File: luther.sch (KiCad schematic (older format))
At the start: 6 parts, among them J1 Conn_01x02, U1 Teensy4.0, U2 RFM95W_LoRa_Radio, U3 VHN5019_Breakout, U4 VHN5019_Breakout, U5 bno055

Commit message: misc changes
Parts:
- removed U5: bno055, NUSTARS Libs:bno055, symbol NUSTARS:bno055
- added D1: LED, symbol Device:LED
- added J2: SMART_AUDIO, symbol Connector_Generic:Conn_01x02
- added J3: SERVO_LEVER, Connector_JST:JST_PH_B3B-PH-K_1x03_P2.00mm_Vertical, symbol Connector_Generic:Conn_01x03
- added J4: SERVO_CLOCK, Connector_JST:JST_PH_B3B-PH-K_1x03_P2.00mm_Vertical, symbol Connector_Generic:Conn_01x03
- added R1: 330, symbol Device:R_Small_US
- added SW1: SW_SPST, NUSTARS Libs:GF-123-0054, symbol Switch:SW_SPST
- added U5: VHN5019_Breakout, NUSTARS Libs:VNH5019_breakout, symbol NUSTARS:VHN5019_Breakout
- added U6, U7: BUCK, symbol NUSTARS:BUCK
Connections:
- net labels added: 3V3B, M0_INA, M0_INB, M0_PWM, M1_INA, M1_INB, M1_PWM, M2_INA, M2_INB, M2_PWM
- net labels removed: FNA2T, T2FNA
- wire segments 5 -> 26
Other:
- note removed: "Consider hooking this up to 3.3V buck output\n"
- moved on the sheet: J1, U2, U3, U4

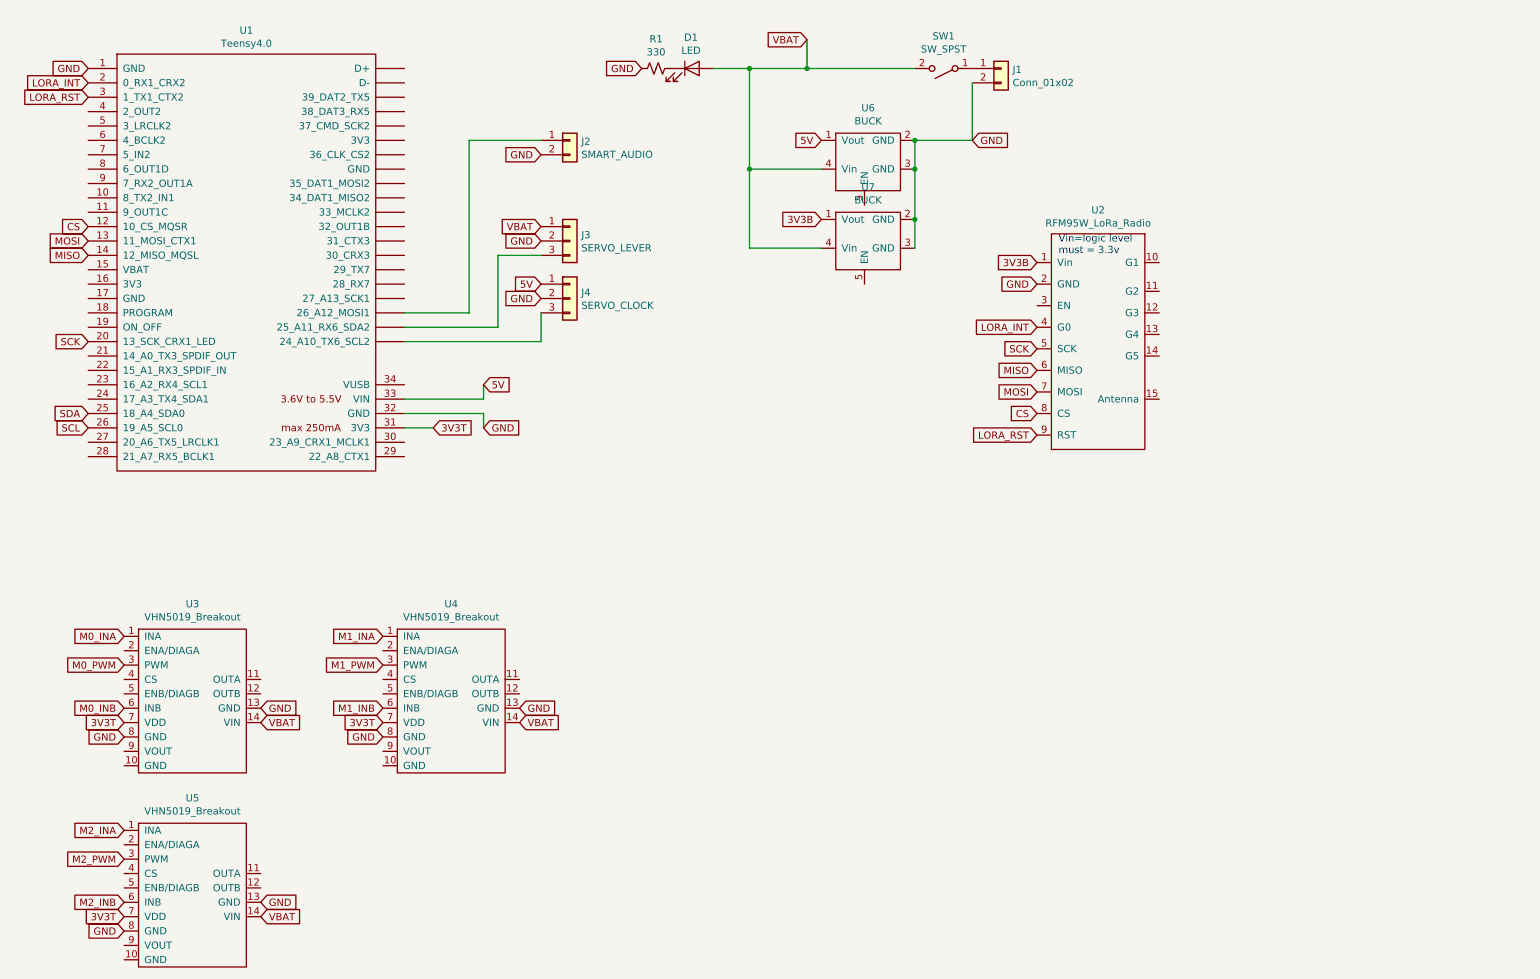
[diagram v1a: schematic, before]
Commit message: updates
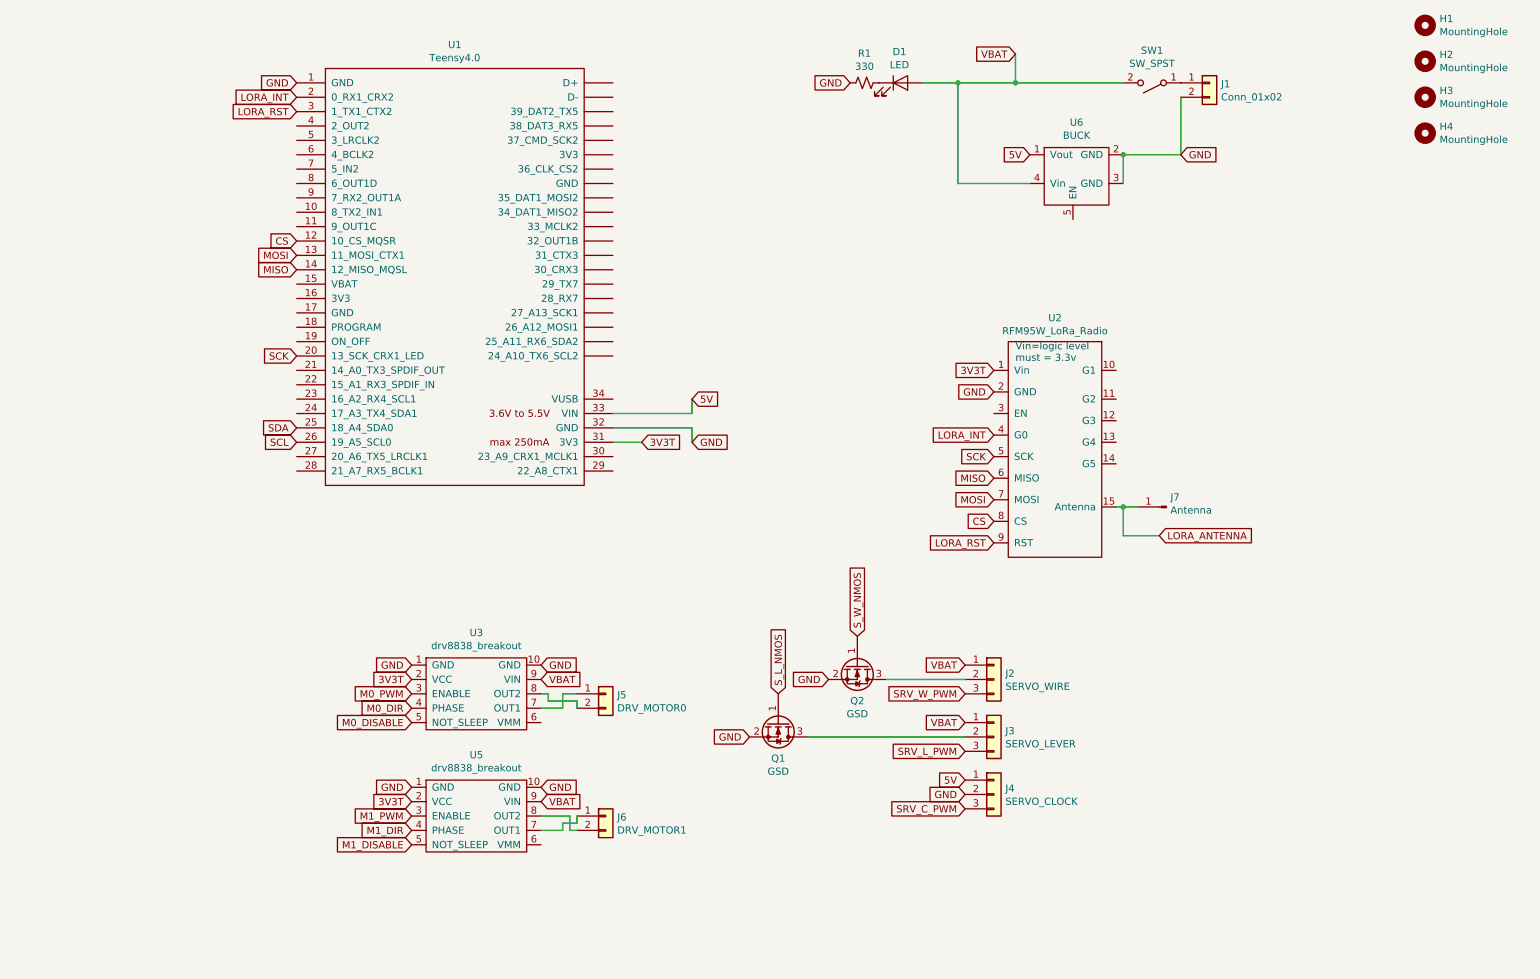
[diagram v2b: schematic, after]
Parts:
- removed J2: SMART_AUDIO, symbol Connector_Generic:Conn_01x02
- removed U3, U4, U5: VHN5019_Breakout, NUSTARS Libs:VNH5019_breakout, symbol NUSTARS:VHN5019_Breakout
- removed U7: BUCK, symbol NUSTARS:BUCK
- added H1, H2, H3, H4: MountingHole, MountingHole:MountingHole_3.2mm_M3, symbol Mechanical:MountingHole
- added J2: SERVO_WIRE, Connector_JST:JST_PH_B3B-PH-K_1x03_P2.00mm_Vertical, symbol Connector_Generic:Conn_01x03
- added J5: DRV_MOTOR0, Connector_JST:JST_PH_B2B-PH-K_1x02_P2.00mm_Vertical, symbol Connector_Generic:Conn_01x02
- added J6: DRV_MOTOR1, Connector_JST:JST_PH_B2B-PH-K_1x02_P2.00mm_Vertical, symbol Connector_Generic:Conn_01x02
- added J7: Antenna, NUSTARS Libs:Antenna, symbol Connector:Conn_01x01_Male
- added Q1, Q2: GSD, Package_TO_SOT_SMD:SOT-23_Handsoldering, symbol Device:Q_NMOS_GSD
- added U3, U5: drv8838_breakout, NUSTARS Libs:drv8838_breakout, symbol DRV:drv8838_breakout
- D1: footprint (none) -> LED_SMD:LED_1206_3216Metric_Pad1.42x1.75mm_HandSolder
- R1: footprint (none) -> Resistor_SMD:R_1206_3216Metric_Pad1.42x1.75mm_HandSolder
- U6: footprint (none) -> NUSTARS Libs:D24V50F5
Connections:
- net 3V3B is gone; now on net 3V3T: U2.1 (Vin)
- net 3V3T: now also U3.2 (VCC), U5.2 (VCC)
- net GND: now also Q1.2 (S), Q2.2 (S), U3.1 (GND), U3.10 (GND), U5.1 (GND), U5.10 (GND); no longer J3.2 (Pin_2)
- net M0_PWM: now also U3.3 (ENABLE)
- net M1_PWM: now also U5.3 (ENABLE)
- net VBAT: now also J2.1 (Pin_1), U3.9 (VIN), U5.9 (VIN)
- net SRV_L_PWM: now reaches J3.3 (Pin_3)
- net SRV_L_PWM: no longer U1.~ (GND)
- net SRV_C_PWM: now reaches J4.3 (Pin_3)
- net SRV_C_PWM: no longer U1.~ (GND)
- net LORA_ANTENNA: now reaches U2.15 (Antenna)
- net LORA_ANTENNA: now also J7.1 (Pin_1)
- new net: J6.1 (Pin_1), U5.7 (OUT1)
- new net: J6.2 (Pin_2), U5.8 (OUT2)
- new net: J5.1 (Pin_1), U3.7 (OUT1)
- new net: J5.2 (Pin_2), U3.8 (OUT2)
- new net: J3.2 (Pin_2), Q1.3 (D)
- new net: J2.2 (Pin_2), Q2.3 (D)
- new net M0_DIR: U3.4 (PHASE)
- new net M0_DISABLE: U3.5 (NOT_SLEEP)
- new net M1_DIR: U5.4 (PHASE)
- new net M1_DISABLE: U5.5 (NOT_SLEEP)
- new net SRV_W_PWM: J2.3 (Pin_3)
- new net S_L_NMOS: Q1.1 (G)
- new net S_W_NMOS: Q2.1 (G)
- now unconnected: U1.~ (GND)
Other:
- moved on the sheet: D1, J1, J3, J4, R1, SW1, U1, U2, U6
